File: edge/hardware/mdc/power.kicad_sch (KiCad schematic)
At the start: 5 parts, among them J2 Screw_Terminal_01x02, J3 Screw_Terminal_01x02, J4 Screw_Terminal_01x02

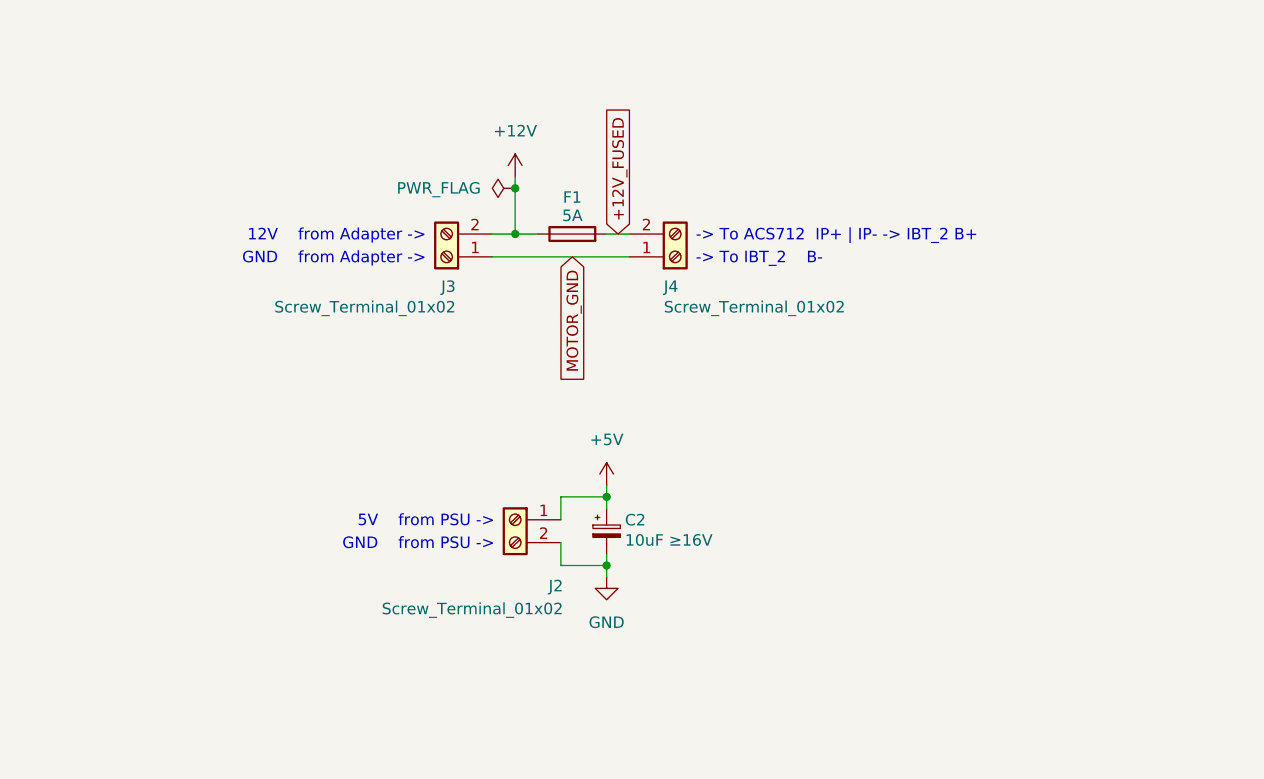
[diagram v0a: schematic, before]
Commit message: update rev3.0 schematic and layout
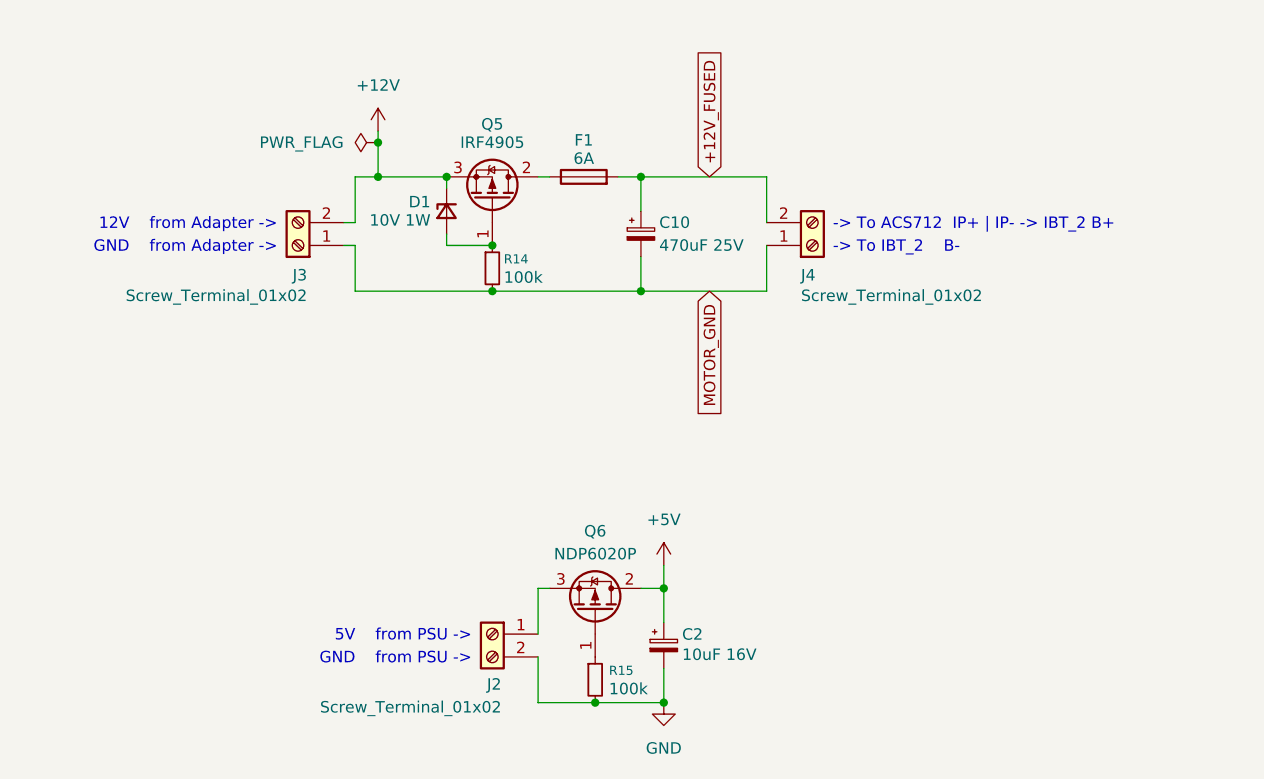
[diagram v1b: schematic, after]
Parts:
- added C10: 470uF 25V, Capacitor_THT:CP_Radial_D5.0mm_P2.50mm, symbol Device:C_Polarized_Small
- added D1: 10V 1W, Diode_THT:D_DO-41_SOD81_P7.62mm_Horizontal, symbol Device:D_Zener_Small
- added Q5: IRF4905, Package_TO_SOT_THT:TO-220-3_Vertical, symbol Transistor_FET:IRF4905
- added Q6: NDP6020P, Package_TO_SOT_THT:TO-220-3_Vertical, symbol Transistor_FET:IRF4905
- added R14, R15: 100k, Resistor_THT:R_Axial_DIN0207_L6.3mm_D2.5mm_P7.62mm_Horizontal, symbol Device:R_Small
- C2: value 10uF ≥16V -> 10uF 16V
- F1: value 5A -> 6A
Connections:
- net +12V: now also D1.1 (K), Q5.3 (S); no longer F1.1
- net +12V_FUSED: now also C10.1
- net +5V: now also Q6.2 (D); no longer J2.1 (Pin_1)
- net GND: now also R15.2
- net MOTOR_GND: now also C10.2, R14.2
- new net: D1.2 (A), Q5.1 (G), R14.1
- new net: J2.1 (Pin_1), Q6.3 (S)
- new net: Q6.1 (G), R15.1
- new net: F1.1, Q5.2 (D)
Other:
- moved on the sheet: C2, F1, J2, J3, J4

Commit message: update rev3.0 schematic and layout
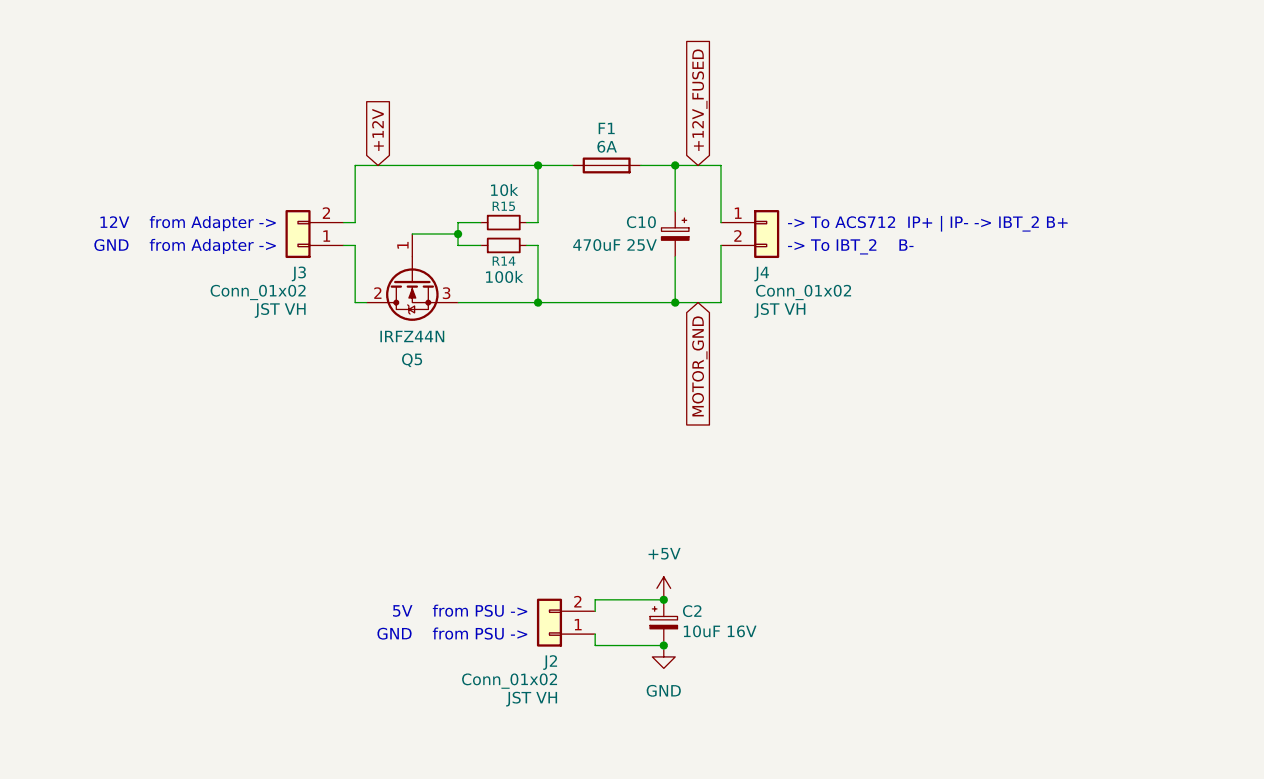
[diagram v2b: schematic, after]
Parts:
- removed D1: 10V 1W, Diode_THT:D_DO-41_SOD81_P7.62mm_Horizontal, symbol Device:D_Zener_Small
- removed J2, J3, J4: Screw_Terminal_01x02, TerminalBlock_Altech:Altech_AK100_1x02_P5.00mm, symbol Connector:Screw_Terminal_01x02
- removed Q5: IRF4905, Package_TO_SOT_THT:TO-220-3_Vertical, symbol Transistor_FET:IRF4905
- removed Q6: NDP6020P, Package_TO_SOT_THT:TO-220-3_Vertical, symbol Transistor_FET:IRF4905
- added J2, J3, J4: Conn_01x02, Connector_JST:JST_VH_B2P-VH-B_1x02_P3.96mm_Vertical, symbol Connector_Generic:Conn_01x02
- added Q5: IRFZ44N, Package_TO_SOT_THT:TO-220-3_Vertical, symbol Transistor_FET:IRF540N
- C10: footprint Capacitor_THT:CP_Radial_D5.0mm_P2.50mm -> Capacitor_THT:CP_Radial_D8.0mm_P3.50mm
- R15: value 100k -> 10k
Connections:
- net +12V: now also F1.1, R15.2, J3.2 (Pin_2)
- net +12V_FUSED: now also J4.1 (Pin_1)
- net +5V: now also J2.2 (Pin_2)
- net GND: now also J2.1 (Pin_1); no longer R15.2
- net MOTOR_GND: now also J4.2 (Pin_2), Q5.3 (S)
- net at R14.1: now also R15.1, Q5.1 (G)
- new net: J3.1 (Pin_1), Q5.2 (D)
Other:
- moved on the sheet: C10, C2, F1, R14
